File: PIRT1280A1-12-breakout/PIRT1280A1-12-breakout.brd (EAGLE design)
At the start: 76.2 x 68.6 mm, 39 parts, among them U1 PIRT1280A1-12

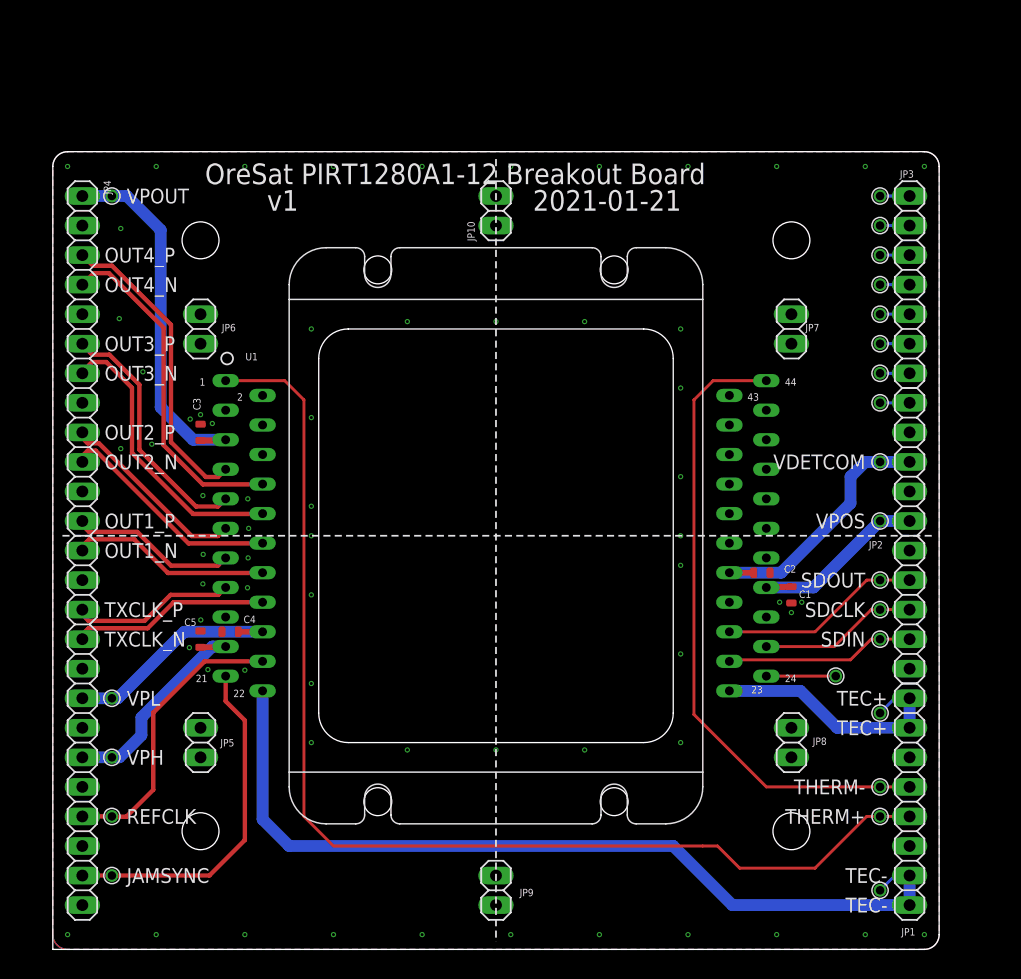
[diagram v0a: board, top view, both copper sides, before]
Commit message: mostly finished PIRT breakout
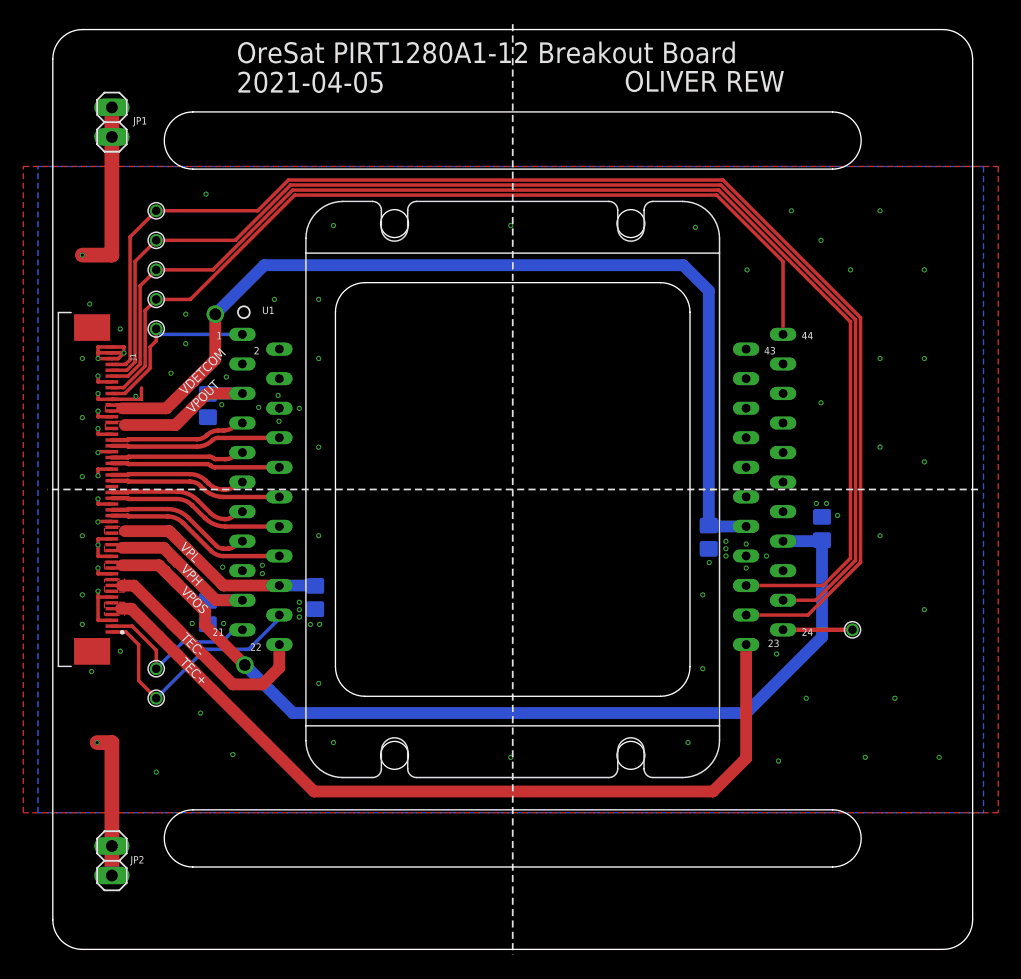
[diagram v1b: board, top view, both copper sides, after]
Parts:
- removed C1, C2, C3, C4, C5: 100n, oresat-rcl:.0603-C-NOSILK
- removed JP10, JP5, JP6, JP7, JP8, JP9: (no value), pinhead:1X02
- removed JP3: (no value), pinhead:1X07
- removed JP4: (no value), pinhead:1X25
- removed TP10, TP11, TP12, TP13, TP14, TP15, TP16, TP17, TP18, TP19, TP2, TP20, TP21, TP22, TP23, TP3, TP4, TP5, TP6, TP7, TP8, TP9: TEST-POINT-LARGE-SQUARE, oresat-misc:1X01
- added C100, C101, C102, C103, C104: 100n, oresat-rcl:.0805-A
- added J1: 5-1734592-0, J-TEConnectivity-X-1734592-X:TE_5-1734592-0
- added JAMSYNC, REFCLK, SDCLK, SDIN, SDOUT, THERM+, THERM-: TEST-POINT-LARGE-SQUARE, oresat-misc:1X01
- added TEC+, TEC-, VDETCOM, VPH, VPL, VPOS, VPOUT: TEST-POINT_SMD-SMD-10SN, oresat-misc:TESTPOINT_SMD-10SN
- JP1: device pinhead:1X08 -> pinhead:1X02
- JP2: device pinhead:1X10 -> pinhead:1X02
- moved JP1 90.1 mm to (5.08, 71.1), turned to 90 degrees
- moved JP2 74.1 mm to (5.08, 7.62), turned to 90 degrees
- moved TP1 4.23 mm to (68.8, 27.5)
- moved U1 4.23 mm to (39.5, 39.5)
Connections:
- removed net N$1: JP2.1, TP2.1
- removed net N$2: JP3.7, TP9.1
- removed net N$3: JP3.6, TP8.1
- removed net N$4: JP3.5, TP7.1
- removed net N$5: JP3.4, TP6.1
- removed net N$6: JP3.3, TP5.1
- removed net N$7: JP3.2, TP4.1
- removed net N$8: JP3.1, TP3.1
- removed net VEDETCOM-2.9V: C2.1, JP2.3, TP17.1, U1.31
- removed net VPH-3.3V: C5.1, JP4.20, TP21.1, U1.19
- removed net VPL-1.6V: C4.1, JP4.18, TP22.1, U1.18
- removed net VPOS-3.3V: C1.1, JP2.5, TP18.1, U1.30
- removed net VPOUT-0.9V: C3.1, JP4.1, TP23.1, U1.5
- new net VDETCOM: C102.1, J1.39, J1.40, U1.31, VDETCOM.TP
- new net VPH: C100.1, J1.15, J1.16, U1.19, VPH.TP
- new net VPL: C101.1, J1.18, J1.19, U1.18, VPL.TP
- new net VPOS: C103.1, J1.12, J1.13, U1.30, VPOS.TP
- new net VPOUT: C104.1, J1.36, J1.37, U1.5, VPOUT.TP
- net GND: now also C100.2, C101.2, C102.2, C103.2, C104.2, J1.11, J1.14, J1.17, J1.20, J1.23, J1.26, J1.29, J1.3, J1.32, J1.35, J1.38, J1.41, J1.44, J1.48, J1.49, J1.50, J1.7, J1.S1, J1.S2, JP1.1, JP1.2, JP2.1; no longer C1.2, C2.2, C3.2, C4.2, C5.2, JP1.3, JP1.6, JP10.1, JP10.2, JP2.10, JP2.4, JP2.6, JP4.11, JP4.14, JP4.17, JP4.19, JP4.2, JP4.21, JP4.23, JP4.25, JP4.5, JP4.8, JP5.1, JP5.2, JP6.1, JP6.2, JP7.1, JP7.2, JP8.1, JP8.2, JP9.1, JP9.2
- net JAMSYNC: now also J1.2, JAMSYNC.1; no longer JP4.24, TP19.1
- net OUT1_N: now also J1.24; no longer JP4.13
- net OUT1_P: now also J1.25; no longer JP4.12
- net OUT2_N: now also J1.27; no longer JP4.10
- net OUT2_P: now also J1.28; no longer JP4.9
- net OUT3_N: now also J1.30; no longer JP4.7
- net OUT3_P: now also J1.31; no longer JP4.6
- net OUT4_N: now also J1.33; no longer JP4.4
- net OUT4_P: now also J1.34; no longer JP4.3
- net REFCLK: now also J1.1, REFCLK.1; no longer JP4.22, TP20.1
- net SDCLK: now also J1.46, SDCLK.1; no longer JP2.8, TP10.1
- net SDIN: now also J1.47, SDIN.1; no longer JP2.9, TP11.1
- net SDOUT: now also J1.45, SDOUT.1; no longer JP2.7, TP12.1
- net TEC+: now also J1.4, J1.5, J1.6, TEC+.TP; no longer JP1.1, JP1.2, TP14.1
- net TEC-: now also J1.10, J1.8, J1.9, TEC-.TP; no longer JP1.7, JP1.8, TP13.1
- net THERM+: now also J1.42, THERM+.1; no longer JP1.5, TP15.1
- net THERM-: now also J1.43, THERM-.1; no longer JP1.4, TP16.1
- net TXCLK_N: now also J1.21; no longer JP4.16
- net TXCLK_P: now also J1.22; no longer JP4.15
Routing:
- net SDIN: track 16.3 -> 114.8 mm
- net SDCLK: track 13.6 -> 108.7 mm
- net SDOUT: track 17.3 -> 109.0 mm
- net VDETCOM: track 0.00 -> 84.6 mm, vias 0 -> 1
- net THERM+: track 99.0 -> 15.4 mm
- net VPOS: track 0.00 -> 81.7 mm, vias 0 -> 1
- net GND: track 0.00 -> 62.9 mm, vias 64 -> 92
- net TEC-: track 75.3 -> 20.0 mm
- net TEC+: track 22.4 -> 73.1 mm
- net VPOUT-0.9V: track 32.1 -> 0.00 mm
- net VEDETCOM-2.9V: track 22.9 -> 0.00 mm
- net THERM-: track 55.1 -> 76.0 mm
- net VPL-1.6V: track 20.0 -> 0.00 mm
- net VPL: track 0.00 -> 19.8 mm
- net VPH-3.3V: track 19.3 -> 0.00 mm
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- added copper zone on layer 1, net TEC+
- added copper zone on layer 1, net TEC-
- added copper zone on layer 1, net VDETCOM
- added copper zone on layer 1, net VPH
- added copper zone on layer 1, net VPL
- added copper zone on layer 1, net VPOS
- added copper zone on layer 1, net VPOUT
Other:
- board size 76.2 x 68.6 mm -> 79.1 x 79.1 mm
- board text added: "2021-04-05"
- board text added: "50 Pos FFC Cable: 0152660535"
- board text added: "OLIVER REW"
- board text removed: "2021-01-21"
- board text removed: "JAMSYNC"
- board text removed: "OUT1_N"
- board text removed: "OUT1_P"
- board text removed: "OUT2_N"
- board text removed: "OUT2_P"
- board text removed: "OUT3_N"
- board text removed: "OUT3_P"
- board text removed: "OUT4_N"
- board text removed: "OUT4_P"
- board text removed: "REFCLK"
- board text removed: "SDCLK"
- board text removed: "SDIN"
- board text removed: "SDOUT"
- board text removed: "TEC+"
- board text removed: "TEC-"
- board text removed: "THERM+"
- board text removed: "THERM-"
- board text removed: "TXCLK_N"
- board text removed: "TXCLK_P"
- board text removed: "VDETCOM"
- board text removed: "VPH"
- board text removed: "VPL"
- board text removed: "VPOS"
- board text removed: "VPOUT"
- board text removed: "v1"
